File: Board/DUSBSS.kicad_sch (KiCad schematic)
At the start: 11 parts, among them Q2 BC857, U5 AP22652W6-7

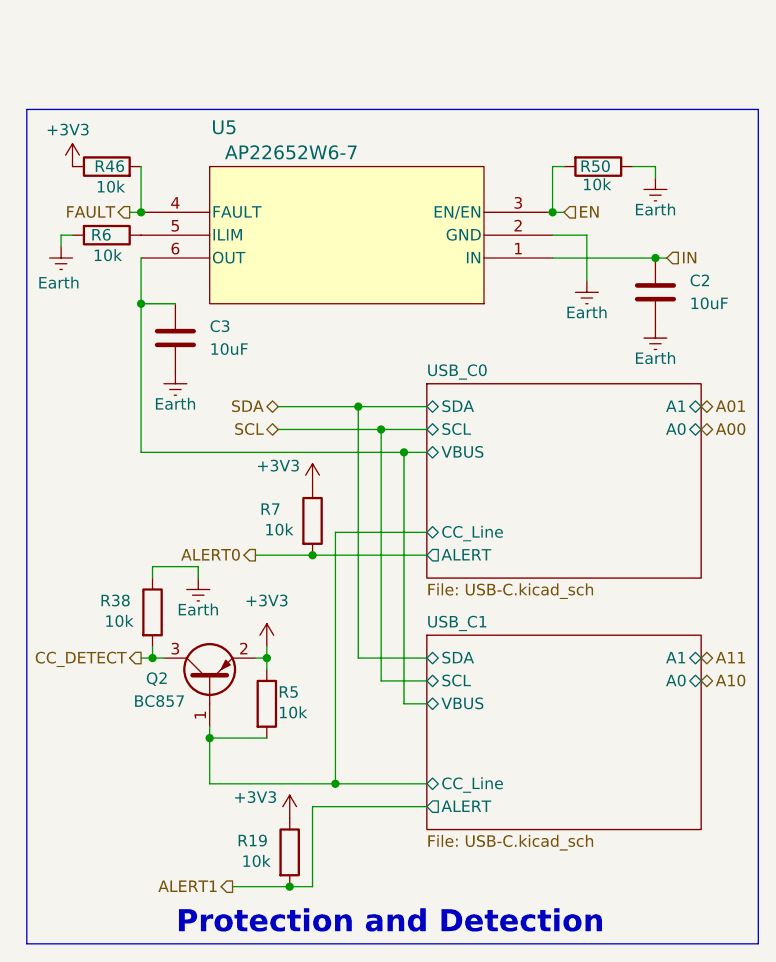
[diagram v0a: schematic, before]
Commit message: Updated documentation
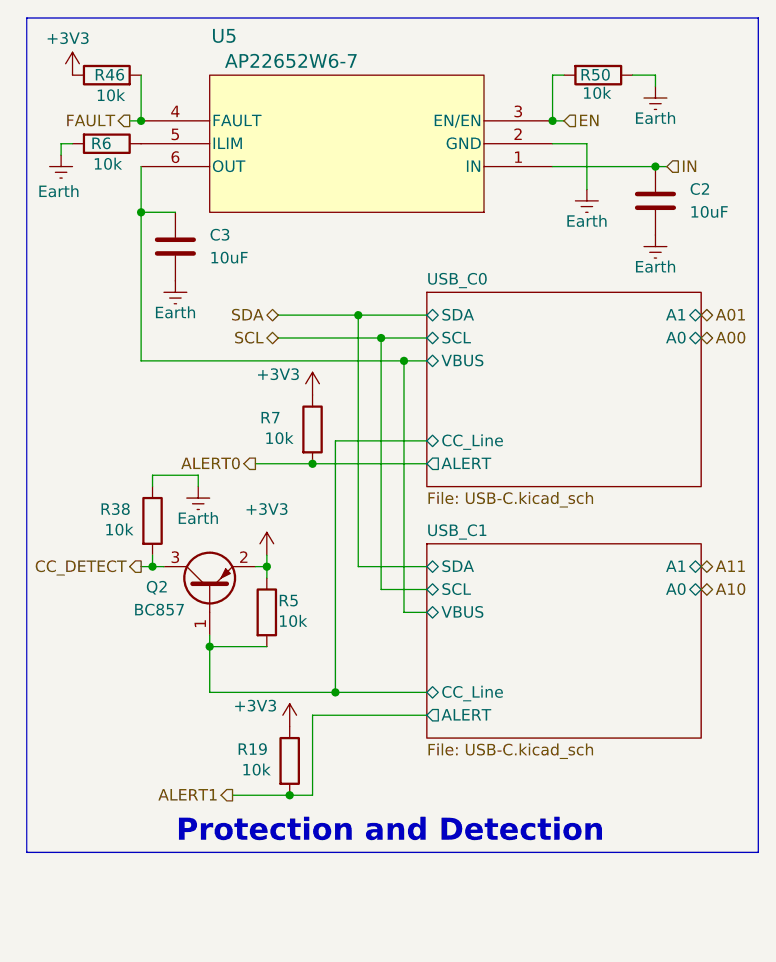
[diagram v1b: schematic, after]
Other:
- moved on the sheet: C2, C3, Q2, R19, R38, R46, R5, R50, R6, R7, U5
